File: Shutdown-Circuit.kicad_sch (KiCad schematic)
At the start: 41 parts, among them Q18 SI2347DS-T1-GE3, Q19 SI2347DS-T1-GE3, Q20 SI2347DS-T1-GE3, Q21 SI2347DS-T1-GE3

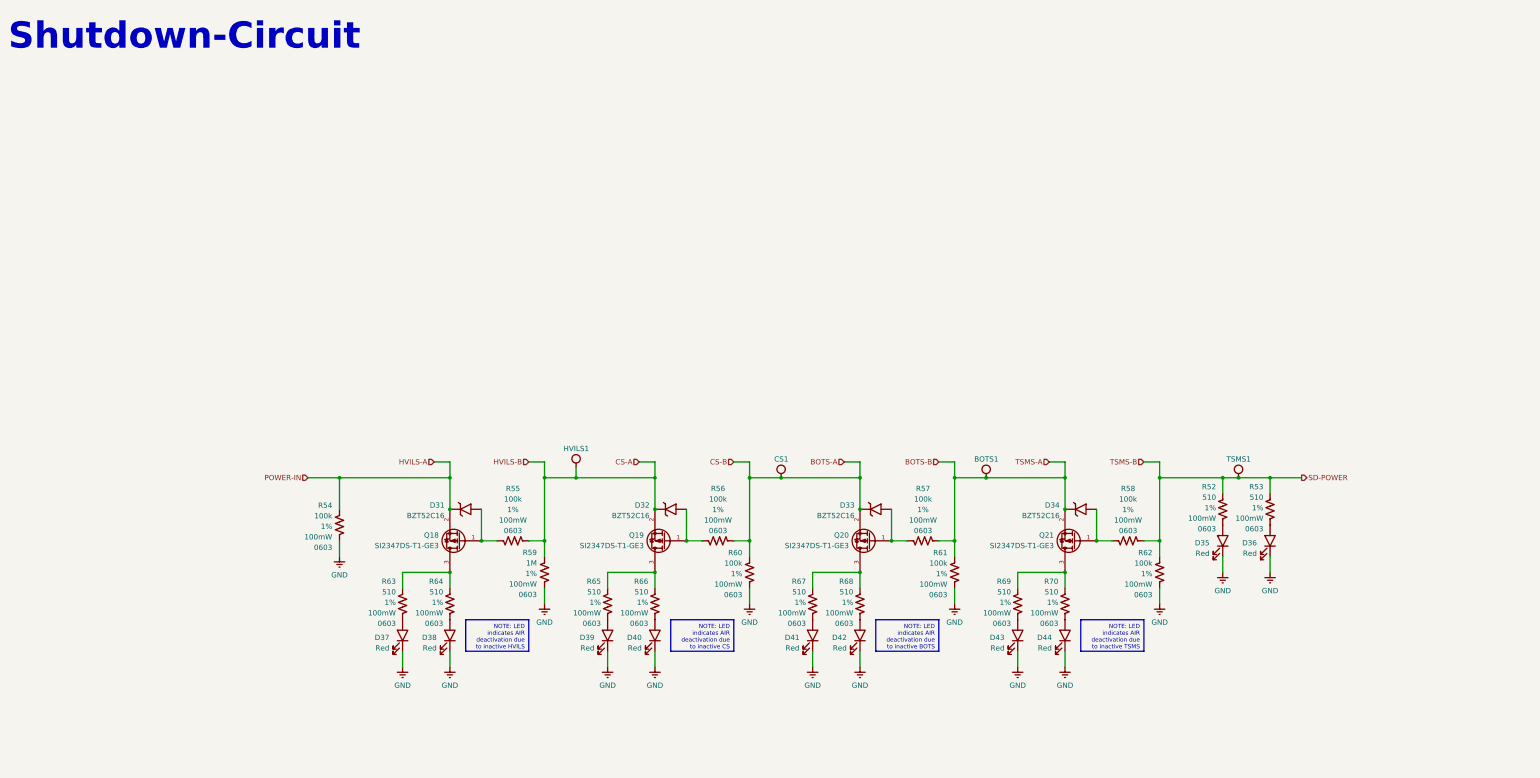
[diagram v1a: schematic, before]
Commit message: schematic updated to V2 extra crispy
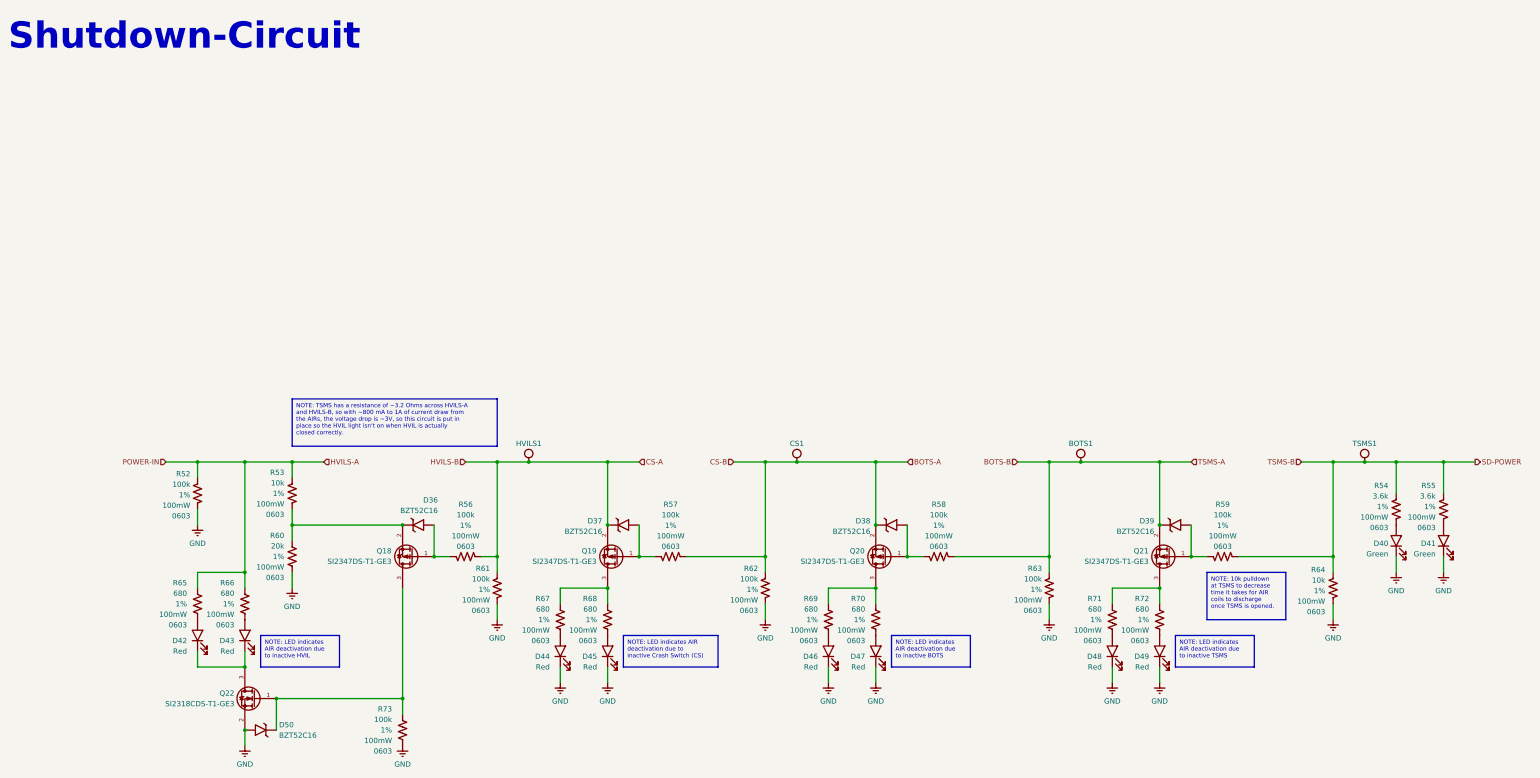
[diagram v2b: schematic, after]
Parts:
- removed D35, D36, D37, D38, D39, D40, D41: Red, LED_SMD:LED_0805_2012Metric, symbol -Diodes-LED:NCD0805R1
- removed R52, R53, R63, R64, R65, R66, R67, R68, R69, R70: 510, Resistor_SMD:R_0603_1608Metric_Pad0.98x0.95mm_HandSolder, symbol -R-SMD-0603:R-0603-510-1%-100mW-100PPM
- removed R59: 1M, Resistor_SMD:R_0603_1608Metric_Pad0.98x0.95mm_HandSolder, symbol -R-SMD-0603:R-0603-1M-1%-100mW-100PPM
- removed R62: 100k, Resistor_SMD:R_0603_1608Metric_Pad0.98x0.95mm_HandSolder, symbol -R-SMD-0603:R-0603-100k-1%-100mW-100PPM
- added D40, D41: Green, LED_SMD:LED_0805_2012Metric, symbol -Diodes-LED:NCD0805G1
- added D45, D46, D47, D48, D49: Red, LED_SMD:LED_0805_2012Metric, symbol -Diodes-LED:NCD0805R1
- added D50: BZT52C16, Diode_SMD:D_SOD-123, symbol -Diodes-Zener:BZT52C16
- added Q22: SI2318CDS-T1-GE3, Package_TO_SOT_SMD:SOT-23-3, symbol -MOSFET-N-Channel:SI2318CDS-T1-GE3
- added R53, R64: 10k, Resistor_SMD:R_0603_1608Metric_Pad0.98x0.95mm_HandSolder, symbol -R-SMD-0603:R-0603-10k-1%-100mW-100PPM
- added R54, R55: 3.6k, Resistor_SMD:R_0603_1608Metric_Pad0.98x0.95mm_HandSolder, symbol -R-SMD-0603:R-0603-3.6k-1%-100mW-100PPM
- added R60: 20k, Resistor_SMD:R_0603_1608Metric_Pad0.98x0.95mm_HandSolder, symbol -R-SMD-0603:R-0603-20k-1%-100mW-100PPM
- added R61, R73: 100k, Resistor_SMD:R_0603_1608Metric_Pad0.98x0.95mm_HandSolder, symbol -R-SMD-0603:R-0603-100k-1%-100mW-100PPM
- added R65, R66, R67, R68, R69, R70, R71, R72: 680, Resistor_SMD:R_0603_1608Metric_Pad0.98x0.95mm_HandSolder, symbol -R-SMD-0603:R-0603-680-1%-100mW-100PPM
- D42, D43, D44: Digikey P/N 350-2039-1-ND -> 160-1427-1-ND; Mouser P/N 645-598-8120-107F -> 859-LTST-C171KRKT
- renumbered D31 to D36, D32 to D37, D33 to D38, D34 to D39, R54 to R52, R55 to R56, R56 to R57, R57 to R58, R58 to R59, R60 to R62, R61 to R63
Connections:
- net CS-A: now also R61.2
- net GND: now also D40.1 (K), D41.1 (K), D45.1 (K), D46.1 (K), D47.1 (K), D48.1 (K), D49.1 (K), D50.2 (A), Q22.2 (S), R60.1, R61.1, R64.1, R73.1; no longer D42.1 (K), D43.1 (K)
- net HVILS-A: now also R53.2, R65.2, R66.2; no longer D36.1 (K), Q18.2 (S)
- net SD-POWER: now also R54.2, R55.2, R64.2
- net at D43.2 (A): now also R66.1
- net at Q20.3 (D): now also R69.2, R70.2
- net at Q18.3 (D): now also D50.1 (K), Q22.1 (G), R73.2
- net at D42.2 (A): now also R65.1
- net at Q19.3 (D): now also R67.2, R68.2
- net at D44.2 (A): now also R67.1
- net at Q21.3 (D): now also R71.2, R72.2
- new net: D36.1 (K), Q18.2 (S), R53.1, R60.2
- new net: D41.2 (A), R55.1
- new net: D45.2 (A), R68.1
- new net: D42.1 (K), D43.1 (K), Q22.3 (D)
- new net: D46.2 (A), R69.1
- new net: D49.2 (A), R72.1
- new net: D40.2 (A), R54.1
- new net: D47.2 (A), R70.1
- new net: D48.2 (A), R71.1
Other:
- moved on the sheet: BOTS1, CS1, D36, D37, D38, D39, HVILS1, Q18, Q19, Q20, Q21, R52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
